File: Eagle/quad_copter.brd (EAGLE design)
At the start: 173.7 x 139.7 mm, 12 parts, among them X1 STM32F4_DISC

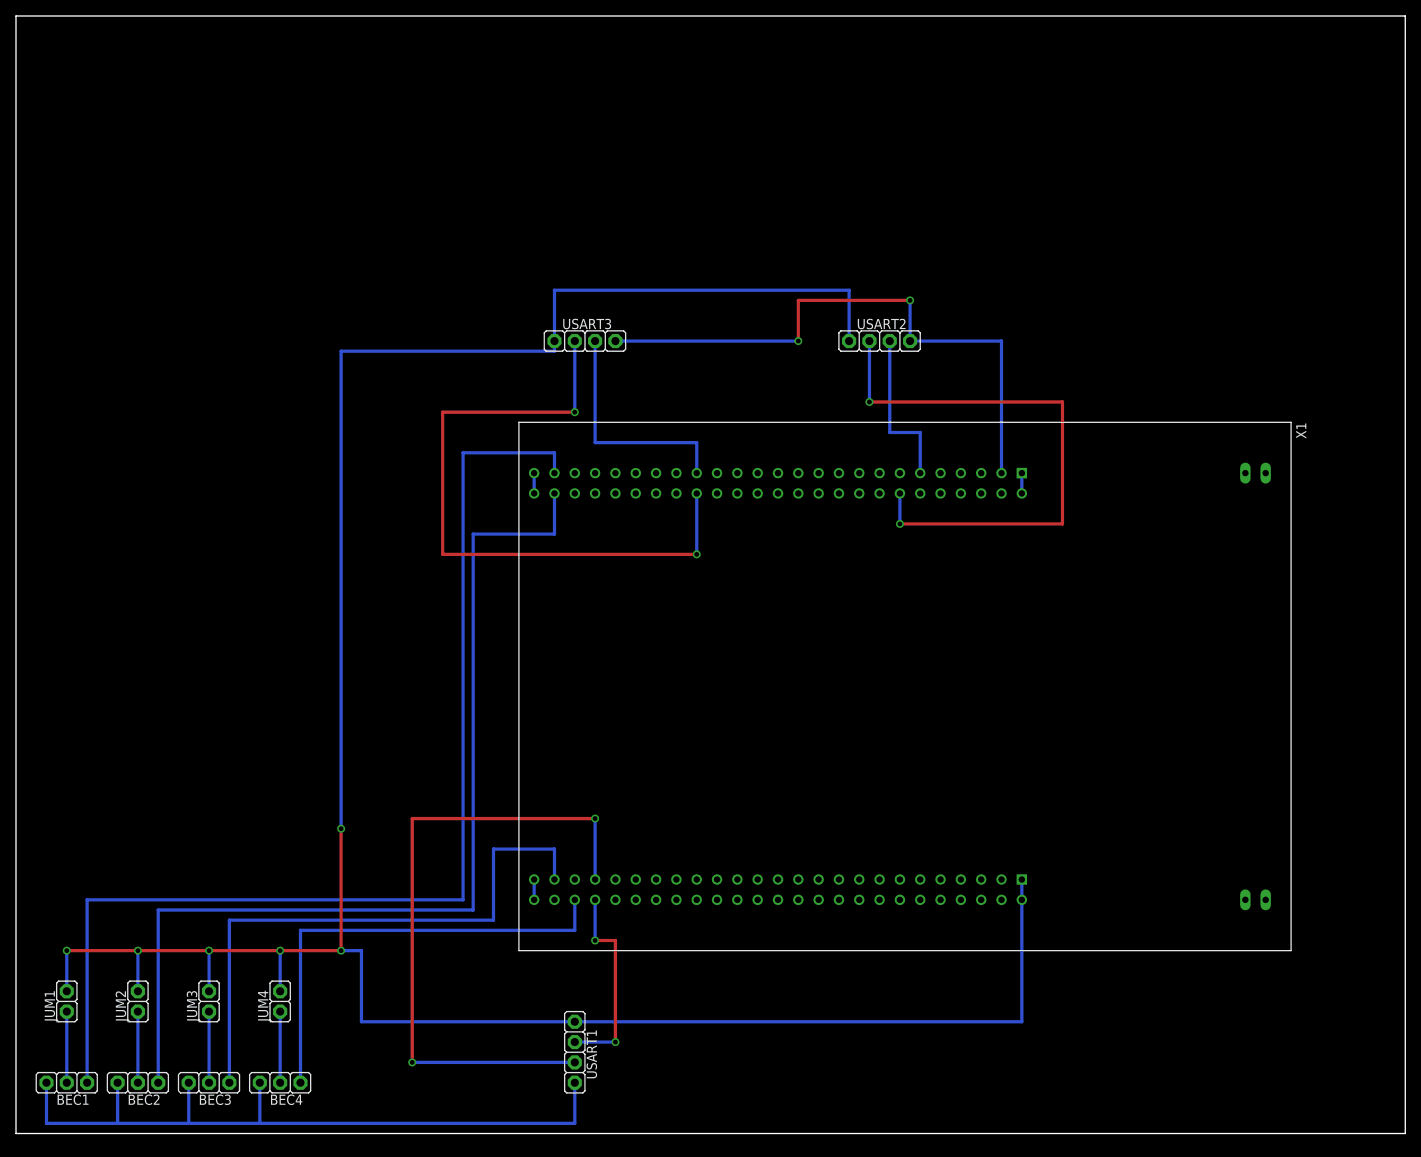
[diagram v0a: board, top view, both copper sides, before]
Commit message: new scheme and board
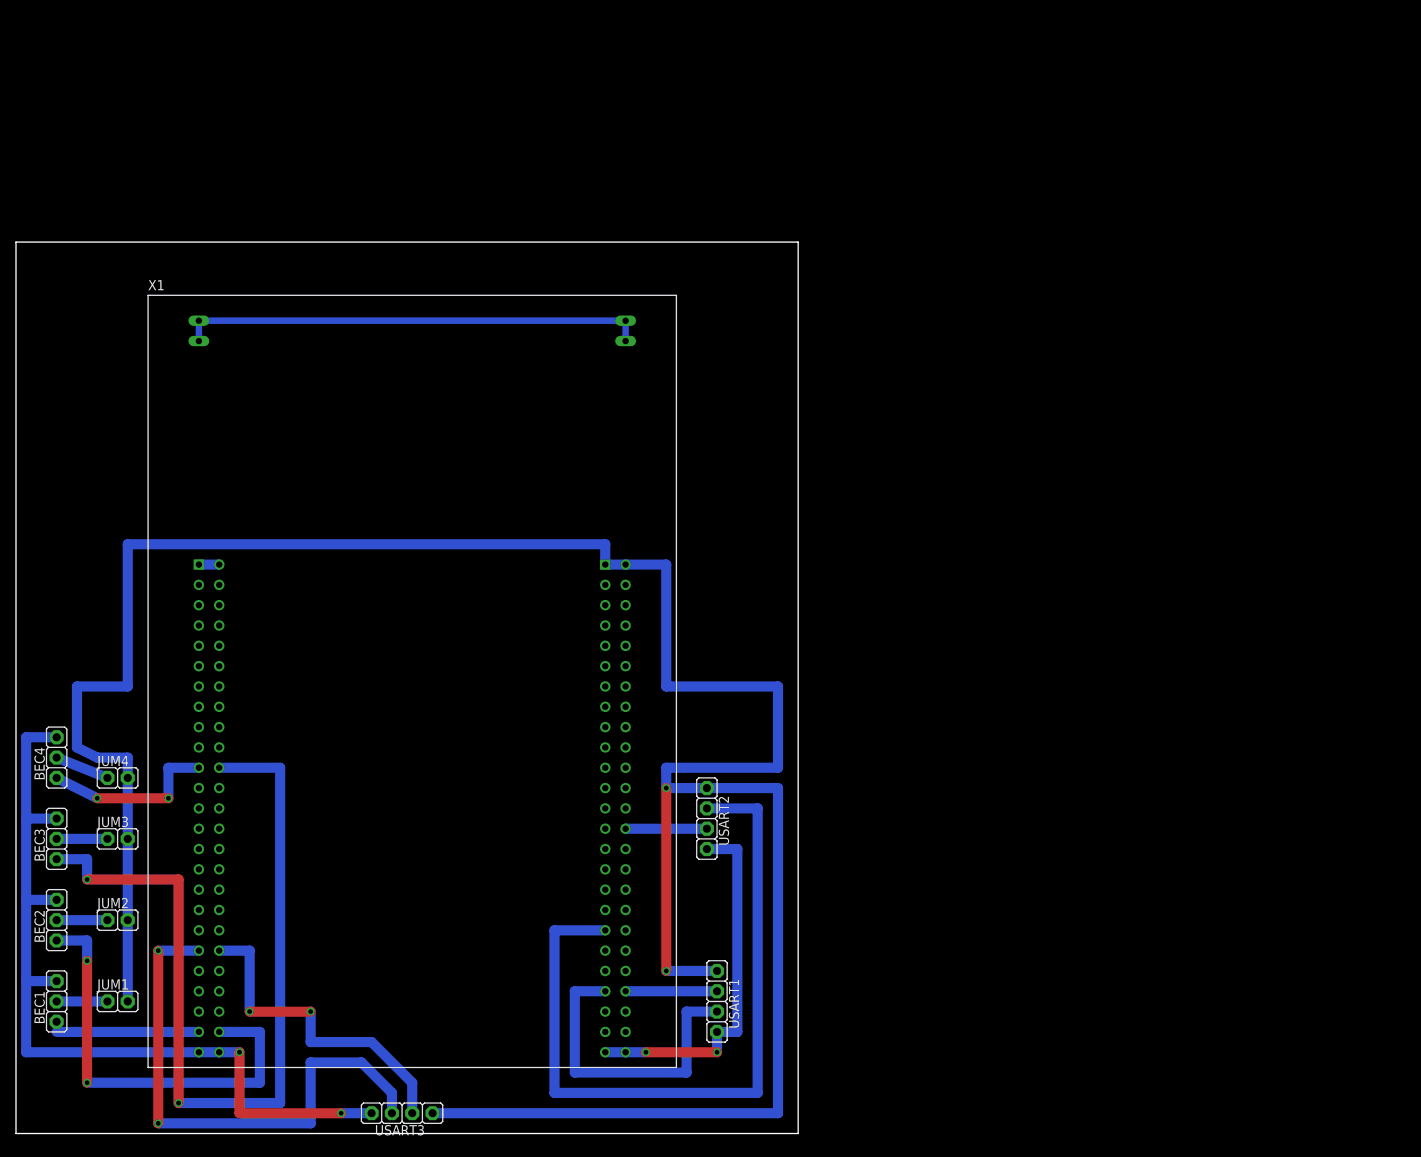
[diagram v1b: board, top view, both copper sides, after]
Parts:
- moved USART3 99.2 mm to (48.3, 2.54), turned to 180 degrees
- moved USART2 63.5 mm to (86.4, 39.4), turned to 270 degrees
- moved BEC4 49.3 mm to (5.08, 47.0), turned to 90 degrees
- moved X1 46.6 mm to (50.8, 40.6), turned to 0 degrees
- moved BEC3 35.9 mm to (5.08, 36.8), turned to 90 degrees
- moved JUM4 34.5 mm to (12.7, 44.5), turned to 0 degrees
- moved JUM3 23.3 mm to (12.7, 36.8), turned to 0 degrees
- moved BEC2 22.7 mm to (5.08, 26.7), turned to 90 degrees
- moved USART1 18.9 mm to (87.6, 16.5)
- moved JUM2 10.5 mm to (12.7, 26.7), turned to 0 degrees
- moved BEC1 10.2 mm to (5.08, 16.5), turned to 90 degrees
- moved JUM1 6.35 mm to (12.7, 16.5), turned to 0 degrees
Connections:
- removed net N$6: USART3.3, X1.L33
- new net N$13: USART2.3, X1.R28
- net 0V: now also X1.L49, X1.L50, X1.R49, X1.R50; no longer X1.T4
- net GND: now also X1.T4; no longer X1.L49, X1.L50, X1.R49, X1.R50
- net N$1: now also USART3.3, X1.L39; no longer USART2.2, X1.L14
- net N$14: now also X1.L21; no longer X1.R46
- net N$15: now also X1.L22; no longer X1.R47
- net N$2: now also USART3.2, X1.L40; no longer USART2.3, X1.L11
- net N$5: now also USART2.2, X1.R37; no longer USART3.2, X1.L34
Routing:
- net N$17: track 139.7 -> 19.1 mm
- net N$16: track 123.2 -> 54.6 mm, vias 0 -> 2
- net GND: track 5.08 -> 58.4 mm
- net N$4: track 81.3 -> 39.4 mm, vias 2 -> 0
- net N$14: track 57.1 -> 22.2 mm, vias 0 -> 2
- net N$15: track 73.7 -> 107.9 mm, vias 0 -> 2
- net N$6: track 29.2 -> 0.00 mm
- net N$2: track 20.3 -> 41.5 mm, vias 0 -> 2
- net 0V: track 166.4 -> 151.1 mm, vias 2 -> 4
- net N$3: track 25.4 -> 11.4 mm, vias 2 -> 0
- net N$5: track 82.5 -> 94.0 mm, vias 2 -> 0
- net N$13: track 0.00 -> 10.2 mm
- net N$1: track 71.1 -> 67.6 mm
- net +5V: track 318.8 -> 321.6 mm, vias 6 -> 2
- net N$12: track 8.89 -> 6.35 mm
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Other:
- board size 173.7 x 139.7 mm -> 97.8 x 111.4 mm
